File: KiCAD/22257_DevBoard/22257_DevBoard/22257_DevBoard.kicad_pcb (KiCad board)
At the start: 6 copper layers, 213.1 x 99.1 mm, 93 parts, among them J1 TD-120-G-AACON40_2X20_TU_HTS_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, J2 TD-120-G-AACON40_2X20_TU_HTS_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, J3 Screw_Terminal_01x02, J4 Conn_Coaxial, J5 Conn_Coaxial, J6 Conn_Coaxial, J7 Conn_Coaxial, U10 74LVC1G17, U11 74LVC1G17, U3 TPS73633DBV, U4 TPS562202, U5 INA219AxD, U6 INA219AxD, U7 BME680, U8 74LVC1G17, U9 74LVC1G17

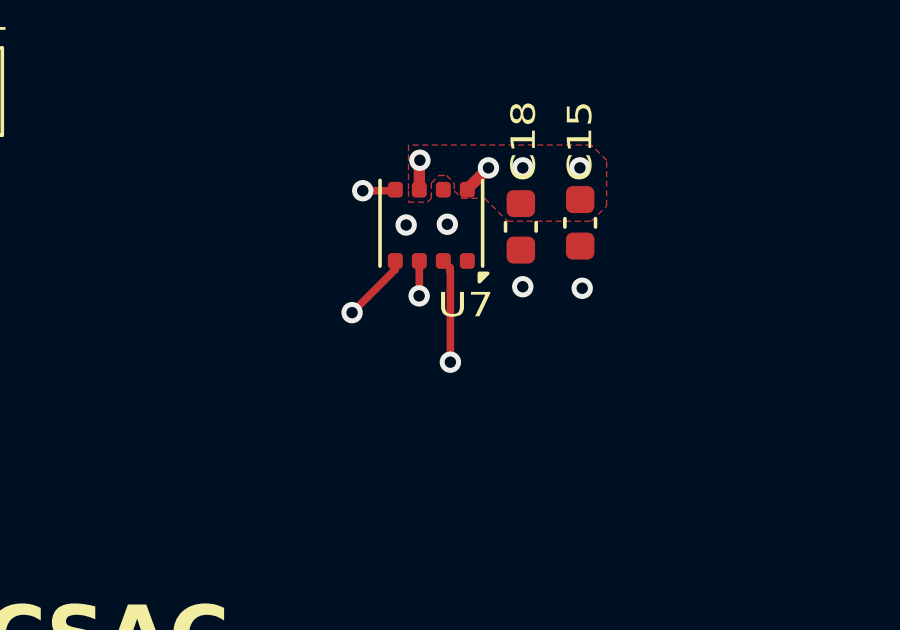
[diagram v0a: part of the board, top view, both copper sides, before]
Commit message: Added notes from review with Carlos
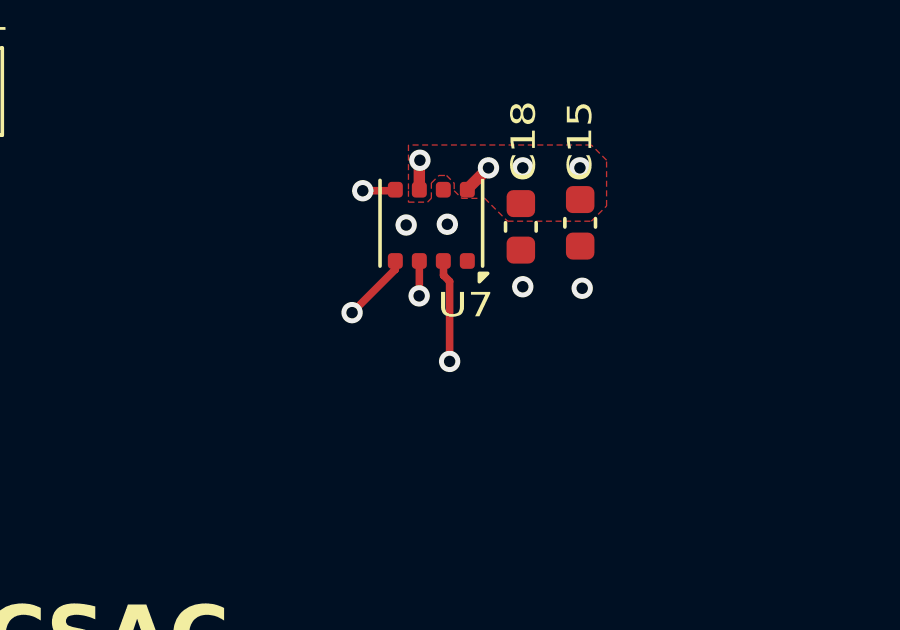
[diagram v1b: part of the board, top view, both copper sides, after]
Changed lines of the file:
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@@
 	)
 	(segment
-		(start 172.085 42.037)
-		(end 172.085 39.005104)
+		(start 171.8564 38.6699)
+		(end 171.85 38.6635)
 		(width 0.254)
 		(layer "F.Cu")
@@
 	)
 	(segment
-		(start 172.085 39.005104)
-		(end 172.072 38.992104)
-		(width 0.254)
-		(layer "F.Cu")
-		(net 24)
-	)
-	(segment
 		(start 61.396828 5.575201)
 		(end 61.396828 14.041172)
@@
 	)
 	(segment
-		(start 172.072 38.8855)
-		(end 171.85 38.6635)
+		(start 172.0596 42.0116)
+		(end 172.0596 39.3446)
 		(width 0.254)
 		(layer "F.Cu")
@@
 	)
 	(segment
-		(start 172.072 38.992104)
-		(end 172.072 38.8855)
+		(start 171.8564 39.1414)
+		(end 171.8564 38.6699)
+		(width 0.254)
+		(layer "F.Cu")
+		(net 24)
+	)
+	(segment
+		(start 172.0596 39.3446)
+		(end 171.8564 39.1414)
 		(width 0.254)
 		(layer "F.Cu")
@@
 	)
 	(via
-		(at 172.085 42.037)
+		(at 172.0596 42.0116)
 		(size 0.7112)
 		(drill 0.381)
@@
 	)
 	(segment
+		(start 162.7632 51.3588)
+		(end 136.398 51.3588)
+		(width 0.254)
+		(layer "In2.Cu")
+		(net 24)
+	)
+	(segment
+		(start 172.0596 42.0624)
+		(end 162.7632 51.3588)
+		(width 0.254)
+		(layer "In2.Cu")
+		(net 24)
+	)
+	(segment
 		(start 136.398 51.3588)
 		(end 134.9248 49.8856)
+		(width 0.254)
+		(layer "In2.Cu")
+		(net 24)
+	)
+	(segment
+		(start 53.4924 18.6436)
+		(end 54.273448 17.862552)
+		(width 0.254)
+		(layer "In2.Cu")
+		(net 24)
+	)
+	(segment
+		(start 53.4924 29.6164)
+		(end 53.4924 18.6436)
 		(width 0.254)
 		(layer "In2.Cu")
@@
 	)
 	(segment
-		(start 162.8648 51.3588)
-		(end 136.398 51.3588)
-		(width 0.254)
-		(layer "In2.Cu")
-		(net 24)
-	)
-	(segment
-		(start 171.8564 42.2656)
-		(end 171.8564 42.3672)
-		(width 0.254)
-		(layer "In2.Cu")
-		(net 24)
-	)
-	(segment
-		(start 53.4924 18.6436)
-		(end 54.273448 17.862552)
-		(width 0.254)
-		(layer "In2.Cu")
-		(net 24)
-	)
-	(segment
-		(start 172.085 42.037)
-		(end 171.8564 42.2656)
-		(width 0.254)
-		(layer "In2.Cu")
-		(net 24)
-	)
-	(segment
-		(start 53.4924 29.6164)
-		(end 53.4924 18.6436)
-		(width 0.254)
-		(layer "In2.Cu")
-		(net 24)
-	)
-	(segment
 		(start 73.7616 49.8856)
 		(end 53.4924 29.6164)
@@
 	)
 	(segment
-		(start 171.8564 42.3672)
-		(end 162.8648 51.3588)
+		(start 172.0596 42.0116)
+		(end 172.0596 42.0624)
 		(width 0.254)
 		(layer "In2.Cu")
